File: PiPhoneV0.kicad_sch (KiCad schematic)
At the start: 44 parts, among them IC1 LM386M-1_NOPB, J1 GPIO, SW1 SW_Push, SW10 SW_Push, SW11 SW_Push, SW12 SW_Push, SW13 SW_Push, SW14 SW_Push, SW15 SW_Push, SW16 SW_Push, SW17 SW_Push, SW18 SW_Push, SW2 SW_Push, SW3 SW_Push, SW4 SW_Push, SW5 SW_Push, SW6 SW_Push, SW7 SW_Push, SW8 SW_Push, SW9 SW_Push

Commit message: chore: body curve
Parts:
- C1, C4: footprint Capacitor_THT:CP_Axial_L10.0mm_D4.5mm_P15.00mm_Horizontal -> Capacitor_SMD:CP_Elec_3x5.3
- C2, C3: footprint Capacitor_THT:CP_Axial_L10.0mm_D4.5mm_P15.00mm_Horizontal -> Capacitor_SMD:C_0201_0603Metric
- D1, D10, D11, D12, D13, D14, D15, D16, D17, D18, D2, D3, D4, D5, D6, D7, D8, D9: footprint Diode_THT:D_5KPW_P12.70mm_Horizontal -> Diode_SMD:D_0201_0603Metric
- R3: footprint Resistor_SMD:R_0201_0603Metric -> Diode_SMD:D_0201_0603Metric
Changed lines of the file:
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@@
 			)
 		)
-		(property "Footprint" "Capacitor_THT:CP_Axial_L10.0mm_D4.5mm_P15.00mm_Horizontal"
+		(property "Footprint" "Capacitor_SMD:CP_Elec_3x5.3"
 			(at 109.22 101.6 0)
 			(effects
@@
 			)
 		)
-		(property "Footprint" "Diode_THT:D_5KPW_P12.70mm_Horizontal"
+		(property "Footprint" "Diode_SMD:D_0201_0603Metric"
 			(at 205.74 102.87 0)
 			(effects
@@
 			)
 		)
-		(property "Footprint" "Diode_THT:D_5KPW_P12.70mm_Horizontal"
+		(property "Footprint" "Diode_SMD:D_0201_0603Metric"
 			(at 205.74 91.44 0)
 			(effects
@@
 			)
 		)
-		(property "Footprint" "Diode_THT:D_5KPW_P12.70mm_Horizontal"
+		(property "Footprint" "Diode_SMD:D_0201_0603Metric"
 			(at 205.74 68.58 0)
 			(effects
@@
 			)
 		)
-		(property "Footprint" "Diode_THT:D_5KPW_P12.70mm_Horizontal"
+		(property "Footprint" "Diode_SMD:D_0201_0603Metric"
 			(at 205.74 80.01 0)
 			(effects
@@
 			)
 		)
-		(property "Footprint" "Resistor_SMD:R_0201_0603Metric"
+		(property "Footprint" "Diode_SMD:D_0201_0603Metric"
 			(at 66.548 121.92 90)
 			(effects
@@
 			)
 		)
-		(property "Footprint" "Diode_THT:D_5KPW_P12.70mm_Horizontal"
+		(property "Footprint" "Diode_SMD:D_0201_0603Metric"
 			(at 165.1 68.58 0)
 			(effects
@@
 			)
 		)
-		(property "Footprint" "Diode_THT:D_5KPW_P12.70mm_Horizontal"
+		(property "Footprint" "Diode_SMD:D_0201_0603Metric"
 			(at 165.1 80.01 0)
 			(effects
@@
 			)
 		)
-		(property "Footprint" "Diode_THT:D_5KPW_P12.70mm_Horizontal"
+		(property "Footprint" "Diode_SMD:D_0201_0603Metric"
 			(at 185.42 45.72 0)
 			(effects
@@
 			)
 		)
-		(property "Footprint" "Diode_THT:D_5KPW_P12.70mm_Horizontal"
+		(property "Footprint" "Diode_SMD:D_0201_0603Metric"
 			(at 165.1 102.87 0)
 			(effects
@@
 			)
 		)
-		(property "Footprint" "Diode_THT:D_5KPW_P12.70mm_Horizontal"
+		(property "Footprint" "Diode_SMD:D_0201_0603Metric"
 			(at 185.42 102.87 0)
 			(effects
@@
 			)
 		)
-		(property "Footprint" "Diode_THT:D_5KPW_P12.70mm_Horizontal"
+		(property "Footprint" "Diode_SMD:D_0201_0603Metric"
 			(at 205.74 45.72 0)
 			(effects
@@
 			)
 		)
-		(property "Footprint" "Diode_THT:D_5KPW_P12.70mm_Horizontal"
+		(property "Footprint" "Diode_SMD:D_0201_0603Metric"
 			(at 165.1 45.72 0)
 			(effects
@@
 			)
 		)
-		(property "Footprint" "Diode_THT:D_5KPW_P12.70mm_Horizontal"
+		(property "Footprint" "Diode_SMD:D_0201_0603Metric"
 			(at 165.1 91.44 0)
 			(effects
@@
 			)
 		)
-		(property "Footprint" "Capacitor_THT:CP_Axial_L10.0mm_D4.5mm_P15.00mm_Horizontal"
+		(property "Footprint" "Capacitor_SMD:CP_Elec_3x5.3"
 			(at 121.92 124.46 0)
 			(effects
@@
 			)
 		)
-		(property "Footprint" "Diode_THT:D_5KPW_P12.70mm_Horizontal"
+		(property "Footprint" "Diode_SMD:D_0201_0603Metric"
 			(at 165.1 57.15 0)
 			(effects
@@
 			)
 		)
-		(property "Footprint" "Capacitor_THT:CP_Axial_L10.0mm_D4.5mm_P15.00mm_Horizontal"
+		(property "Footprint" "Capacitor_SMD:C_0201_0603Metric"
 			(at 117.1448 107.95 0)
 			(effects
@@
 			)
 		)
-		(property "Footprint" "Diode_THT:D_5KPW_P12.70mm_Horizontal"
+		(property "Footprint" "Diode_SMD:D_0201_0603Metric"
 			(at 185.42 91.44 0)
 			(effects
@@
 			)
 		)
-		(property "Footprint" "Capacitor_THT:CP_Axial_L10.0mm_D4.5mm_P15.00mm_Horizontal"
+		(property "Footprint" "Capacitor_SMD:C_0201_0603Metric"
 			(at 112.7252 132.08 0)
 			(effects
@@
 			)
 		)
-		(property "Footprint" "Diode_THT:D_5KPW_P12.70mm_Horizontal"
+		(property "Footprint" "Diode_SMD:D_0201_0603Metric"
 			(at 185.42 68.58 0)
 			(effects
@@
 			)
 		)
-		(property "Footprint" "Diode_THT:D_5KPW_P12.70mm_Horizontal"
+		(property "Footprint" "Diode_SMD:D_0201_0603Metric"
 			(at 205.74 57.15 0)
 			(effects
@@
 			)
 		)
-		(property "Footprint" "Diode_THT:D_5KPW_P12.70mm_Horizontal"
+		(property "Footprint" "Diode_SMD:D_0201_0603Metric"
 			(at 185.42 57.15 0)
 			(effects
@@
 			)
 		)
-		(property "Footprint" "Diode_THT:D_5KPW_P12.70mm_Horizontal"
+		(property "Footprint" "Diode_SMD:D_0201_0603Metric"
 			(at 185.42 80.01 0)
 			(effects

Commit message: fix: switch key switches for low profile
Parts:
- SW1, SW10, SW11, SW12, SW13, SW14, SW15, SW16, SW17, SW18, SW2, SW3, SW4, SW5, SW6, SW7, SW8, SW9: footprint PCM_Switch_Keyboard_Cherry_MX:SW_Cherry_MX_PCB -> 1 key-switches.pretty:SW_MX_LowProfile_THT
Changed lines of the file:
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@@
 			)
 		)
-		(property "Footprint" "PCM_Switch_Keyboard_Cherry_MX:SW_Cherry_MX_PCB"
+		(property "Footprint" "1 key-switches.pretty:SW_MX_LowProfile_THT"
 			(at 157.48 82.55 0)
 			(effects
@@
 			)
 		)
-		(property "Footprint" "PCM_Switch_Keyboard_Cherry_MX:SW_Cherry_MX_PCB"
+		(property "Footprint" "1 key-switches.pretty:SW_MX_LowProfile_THT"
 			(at 177.8 59.69 0)
 			(effects
@@
 			)
 		)
-		(property "Footprint" "PCM_Switch_Keyboard_Cherry_MX:SW_Cherry_MX_PCB"
+		(property "Footprint" "1 key-switches.pretty:SW_MX_LowProfile_THT"
 			(at 198.12 93.98 0)
 			(effects
@@
 			)
 		)
-		(property "Footprint" "PCM_Switch_Keyboard_Cherry_MX:SW_Cherry_MX_PCB"
+		(property "Footprint" "1 key-switches.pretty:SW_MX_LowProfile_THT"
 			(at 177.8 93.98 0)
 			(effects
@@
 			)
 		)
-		(property "Footprint" "PCM_Switch_Keyboard_Cherry_MX:SW_Cherry_MX_PCB"
+		(property "Footprint" "1 key-switches.pretty:SW_MX_LowProfile_THT"
 			(at 198.12 71.12 0)
 			(effects
@@
 			)
 		)
-		(property "Footprint" "PCM_Switch_Keyboard_Cherry_MX:SW_Cherry_MX_PCB"
+		(property "Footprint" "1 key-switches.pretty:SW_MX_LowProfile_THT"
 			(at 177.8 71.12 0)
 			(effects
@@
 			)
 		)
-		(property "Footprint" "PCM_Switch_Keyboard_Cherry_MX:SW_Cherry_MX_PCB"
+		(property "Footprint" "1 key-switches.pretty:SW_MX_LowProfile_THT"
 			(at 157.48 36.83 0)
 			(effects
@@
 			)
 		)
-		(property "Footprint" "PCM_Switch_Keyboard_Cherry_MX:SW_Cherry_MX_PCB"
+		(property "Footprint" "1 key-switches.pretty:SW_MX_LowProfile_THT"
 			(at 177.8 48.26 0)
 			(effects
@@
 			)
 		)
-		(property "Footprint" "PCM_Switch_Keyboard_Cherry_MX:SW_Cherry_MX_PCB"
+		(property "Footprint" "1 key-switches.pretty:SW_MX_LowProfile_THT"
 			(at 198.12 59.69 0)
 			(effects
@@
 			)
 		)
-		(property "Footprint" "PCM_Switch_Keyboard_Cherry_MX:SW_Cherry_MX_PCB"
+		(property "Footprint" "1 key-switches.pretty:SW_MX_LowProfile_THT"
 			(at 177.8 82.55 0)
 			(effects
@@
 			)
 		)
-		(property "Footprint" "PCM_Switch_Keyboard_Cherry_MX:SW_Cherry_MX_PCB"
+		(property "Footprint" "1 key-switches.pretty:SW_MX_LowProfile_THT"
 			(at 177.8 36.83 0)
 			(effects
@@
 			)
 		)
-		(property "Footprint" "PCM_Switch_Keyboard_Cherry_MX:SW_Cherry_MX_PCB"
+		(property "Footprint" "1 key-switches.pretty:SW_MX_LowProfile_THT"
 			(at 198.12 82.55 0)
 			(effects
@@
 			)
 		)
-		(property "Footprint" "PCM_Switch_Keyboard_Cherry_MX:SW_Cherry_MX_PCB"
+		(property "Footprint" "1 key-switches.pretty:SW_MX_LowProfile_THT"
 			(at 157.48 71.12 0)
 			(effects
@@
 			)
 		)
-		(property "Footprint" "PCM_Switch_Keyboard_Cherry_MX:SW_Cherry_MX_PCB"
+		(property "Footprint" "1 key-switches.pretty:SW_MX_LowProfile_THT"
 			(at 157.48 93.98 0)
 			(effects
@@
 			)
 		)
-		(property "Footprint" "PCM_Switch_Keyboard_Cherry_MX:SW_Cherry_MX_PCB"
+		(property "Footprint" "1 key-switches.pretty:SW_MX_LowProfile_THT"
 			(at 157.48 48.26 0)
 			(effects
@@
 			)
 		)
-		(property "Footprint" "PCM_Switch_Keyboard_Cherry_MX:SW_Cherry_MX_PCB"
+		(property "Footprint" "1 key-switches.pretty:SW_MX_LowProfile_THT"
 			(at 157.48 59.69 0)
 			(effects
@@
 			)
 		)
-		(property "Footprint" "PCM_Switch_Keyboard_Cherry_MX:SW_Cherry_MX_PCB"
+		(property "Footprint" "1 key-switches.pretty:SW_MX_LowProfile_THT"
 			(at 198.12 36.83 0)
 			(effects
@@
 			)
 		)
-		(property "Footprint" "PCM_Switch_Keyboard_Cherry_MX:SW_Cherry_MX_PCB"
+		(property "Footprint" "1 key-switches.pretty:SW_MX_LowProfile_THT"
 			(at 198.12 48.26 0)
 			(effects

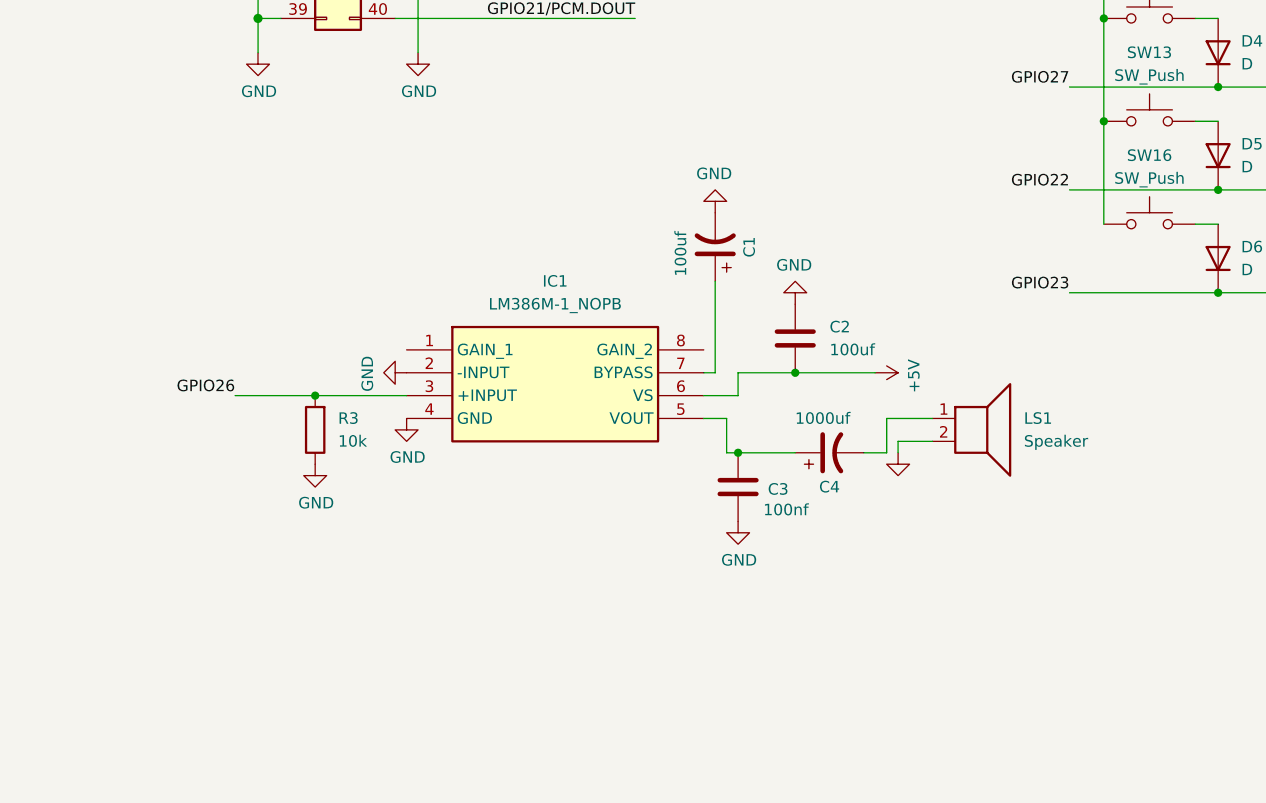
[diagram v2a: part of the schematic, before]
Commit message: feat: routing
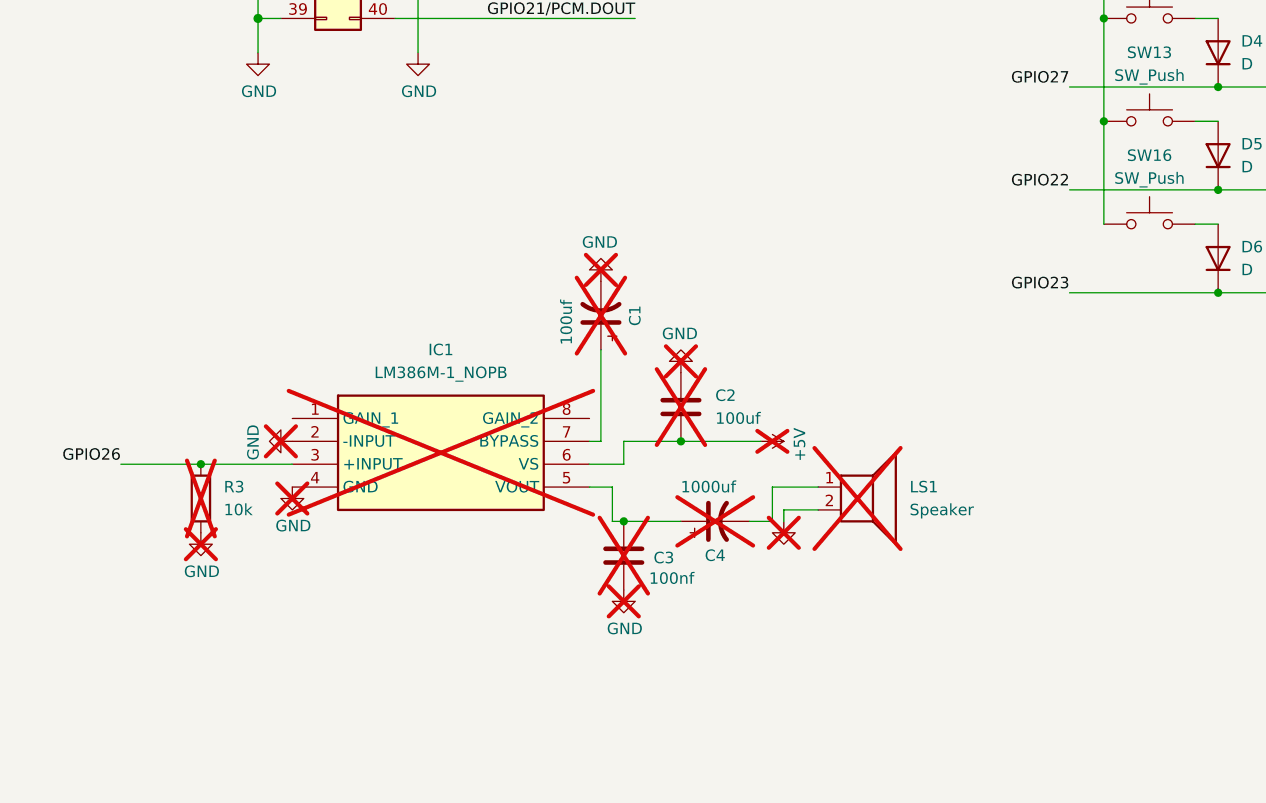
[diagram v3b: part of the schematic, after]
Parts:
- C1, C2, C3, C4, IC1, LS1, R3: now not fitted
